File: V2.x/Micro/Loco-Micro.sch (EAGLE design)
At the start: 30 parts, among them IC1 ATtiny25-20SSH, IC3 MCP1703CB, U1 MCP2551-X/SNSOIC8-N_MC_MCH-L

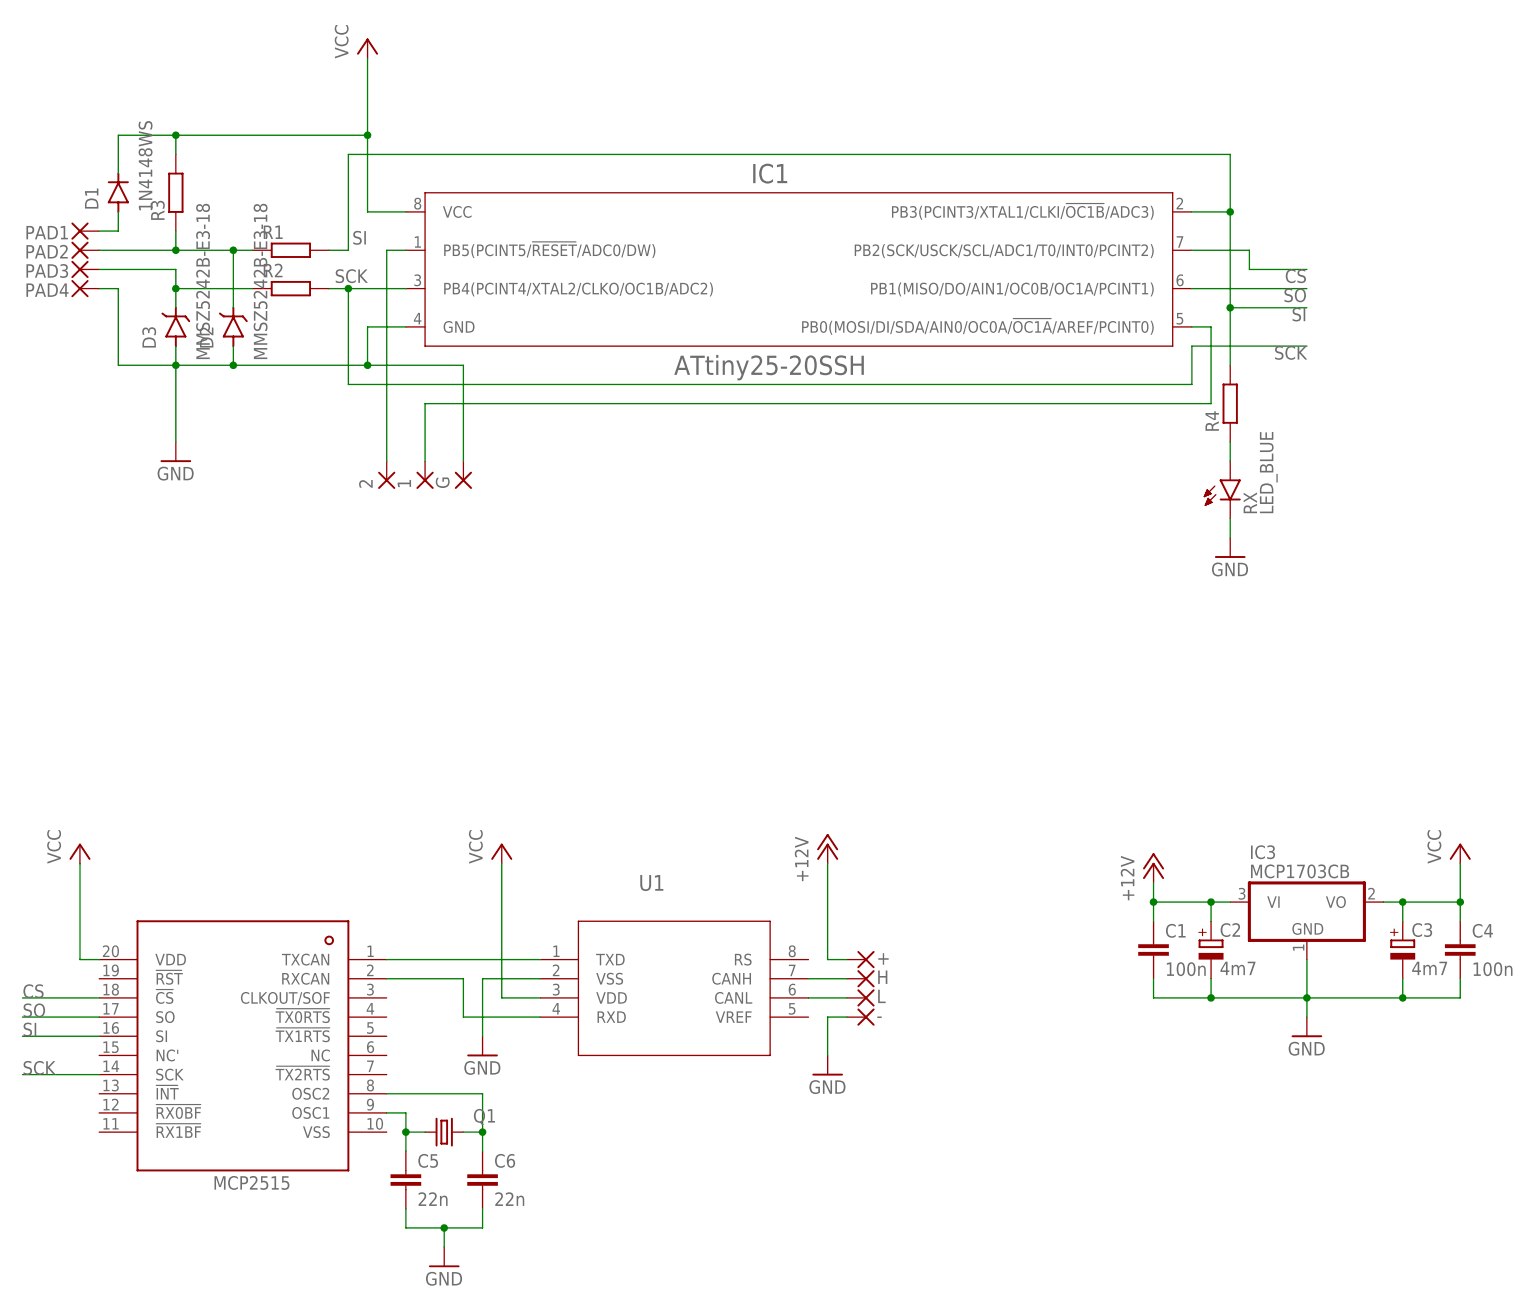
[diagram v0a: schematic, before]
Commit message: updated micro module
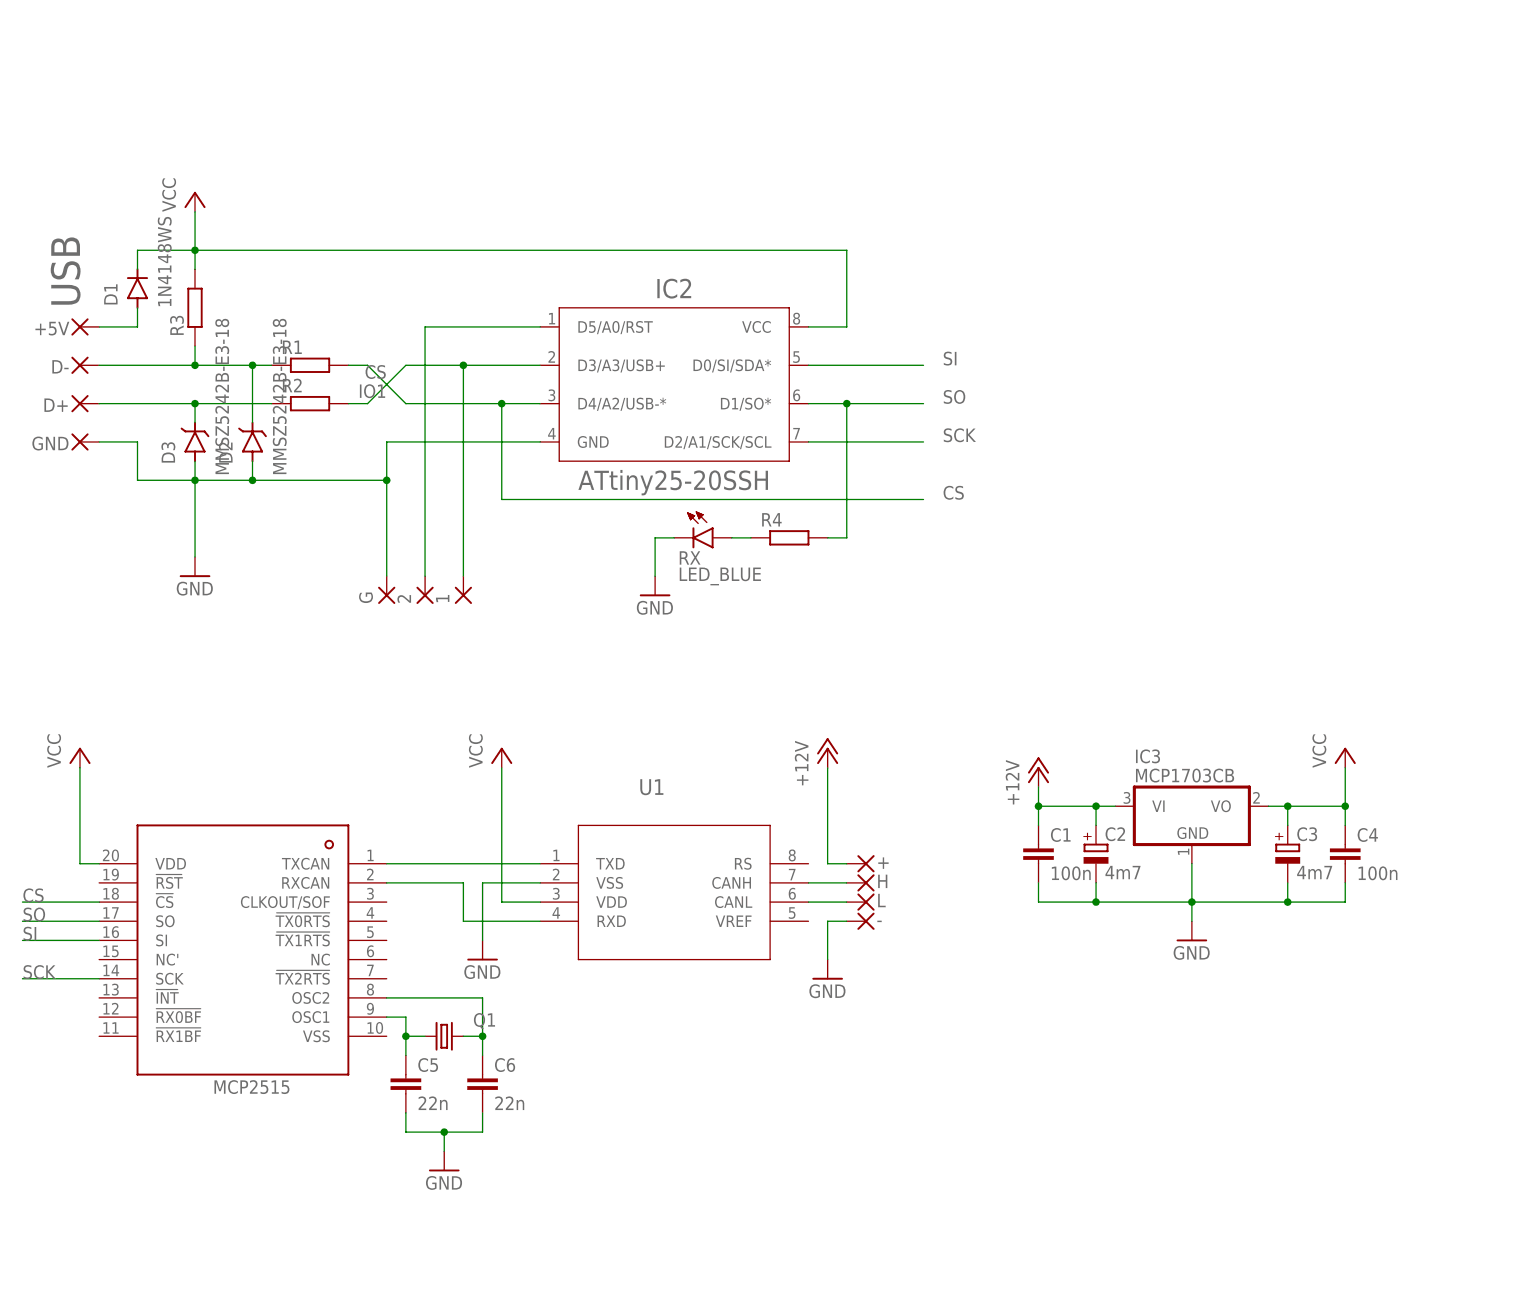
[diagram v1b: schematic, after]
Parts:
- removed IC1: ATtiny25-20SSH, IC_Embedded:ATTINY25-20SSH-8PIN_SOIC
- removed PAD1, PAD2, PAD3, PAD4: (no value), wirepad:SMD2
- added +5V, D+, D-, GND: (no value), wirepad:SMD2
- added IC2: ATtiny25-20SSH, ATtiny:ATTINY25-20SSH-8PIN_SOIC
- C2, C3: device rcl:CPOL-EUA/3216-18W -> rcl:CPOL-EUCT3216
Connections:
- net CS: now also IC2.D4/A2/USB-*, R1.2; no longer IC1.PB2(SCK/USCK/SCL/ADC1/T0/INT0/PCINT2)
- net GND: now also GND.P, IC2.GND; no longer IC1.GND, PAD4.P
- net IO1: now also IC2.D3/A3/USB+, R2.2; no longer IC1.PB0(MOSI/DI/SDA/AIN0/OC0A/!OC1A!/AREF/PCINT0)
- net IO2: now also IC2.D5/A0/RST; no longer IC1.PB5(PCINT5/!RESET!/ADC0/DW)
- net SCK: now also IC2.D2/A1/SCK/SCL; no longer IC1.PB4(PCINT4/XTAL2/CLKO/OC1B/ADC2), R2.2
- net SI: now also IC2.D0/SI/SDA*; no longer IC1.PB3(PCINT3/XTAL1/CLKI/!OC1B!/ADC3), R1.2, R4.2
- net SO: now also IC2.D1/SO*, R4.2; no longer IC1.PB1(MISO/DO/AIN1/OC0B/OC1A/PCINT1)
- net USB_5V: now also +5V.P; no longer PAD1.P
- net USB_D+: now also D+.P; no longer PAD3.P
- net USB_D-: now also D-.P; no longer PAD2.P
- net VCC: now also IC2.VCC; no longer IC1.VCC
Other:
- note added: "USB"
- moved on the sheet: +, -, 1, 2, C1, C2, C3, C4, C5, C6, D1, D2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
